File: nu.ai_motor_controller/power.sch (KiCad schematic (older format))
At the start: 22 parts, among them U5 LMR23625CFDDAR

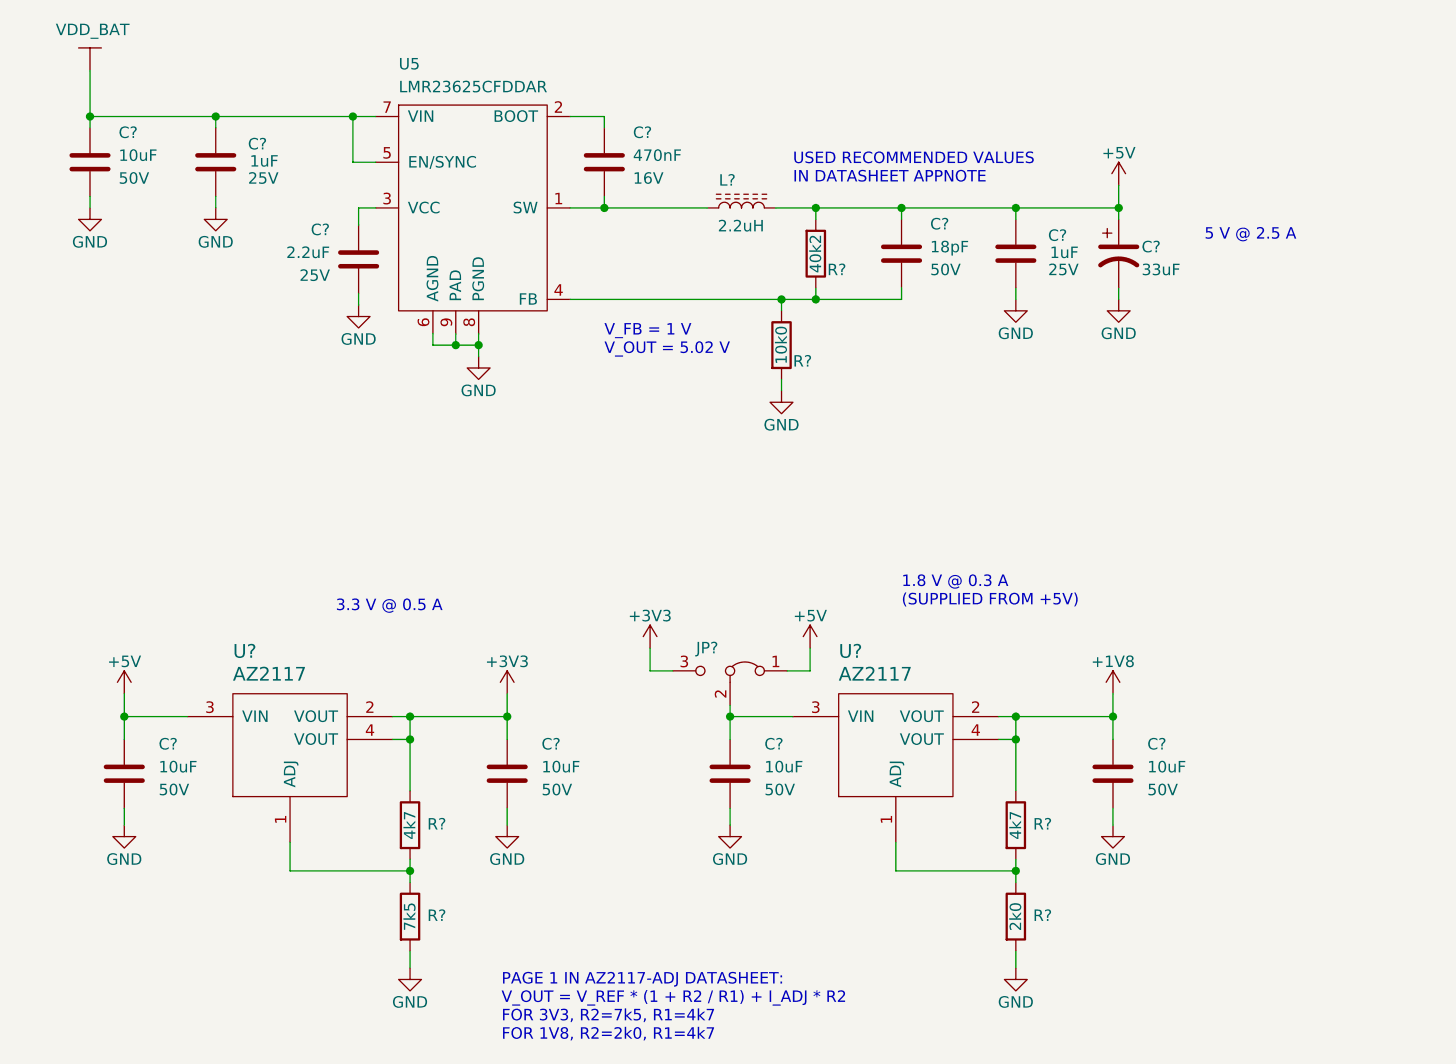
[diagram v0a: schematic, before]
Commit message: automated commit
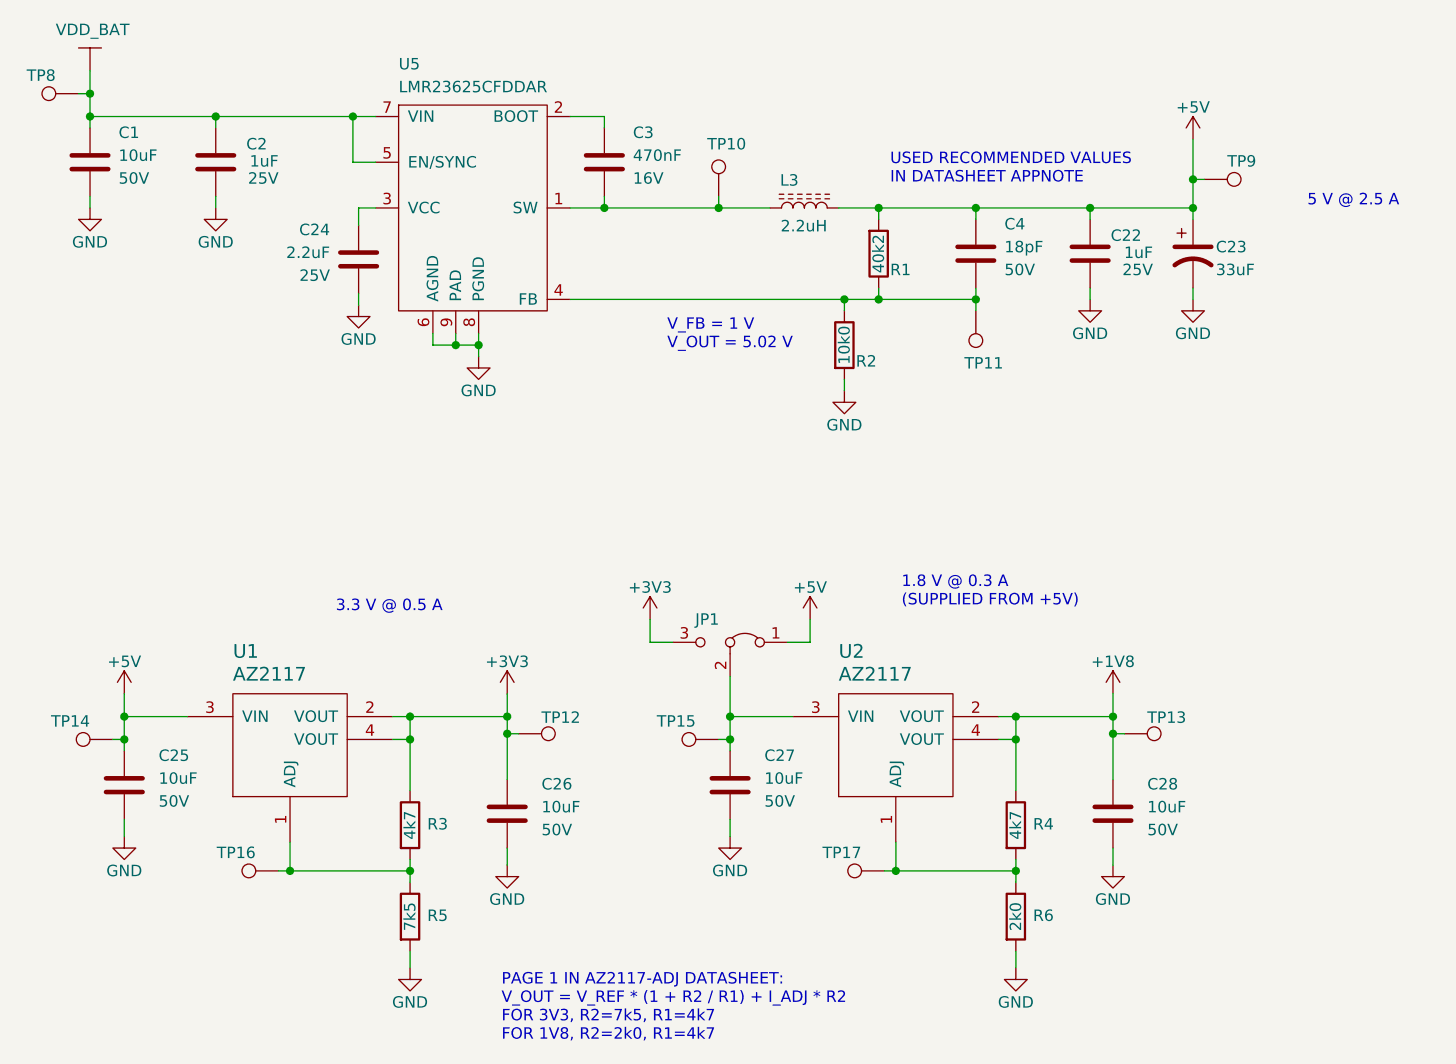
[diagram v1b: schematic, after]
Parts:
- added TP10, TP11, TP12, TP13, TP14, TP15, TP16, TP17, TP8, TP9: PTH_0.5_mm, symbol custom:PTH_0.5_mm
- gave numbers to parts that had none: 21
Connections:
- net +1V8: now also TP13.1
- net +3V3: now also TP12.1
- net +5V: now also TP14.1, TP9.1
- net VDD_BAT: now also TP8.1
- net at C3.2, L3.1, U5.1 (SW): now also TP10.1
- net at C4.2, R1.2, R2.1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: now also TP11.1
- net at R3.2, R5.1, U1.1 (ADJ): now also TP16.1
- net at R4.2, R6.1, U2.1 (ADJ): now also TP17.1
- net at C27.1, JP1.2 (C), U2.3 (VIN): now also TP15.1
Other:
- moved on the sheet: C22, C23, C25, C26, C27, C28, C4, JP1, L3, R1, R2
